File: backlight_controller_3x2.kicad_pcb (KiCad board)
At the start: 2 copper layers, 70.5 x 41.9 mm, 40 parts, among them J1 DB9F_SMD, J2 DB9M_SMD, J3 M12-5-RCPT_F_SMD, J4 M12-5-RCPT_F_SMD, P1 MINI_FIT_JR_02X03_M_RA, U1 SN74ABT541BDWR, U2 SN74ABT541BDWR, U3 NUD3124, U4 NUD3124

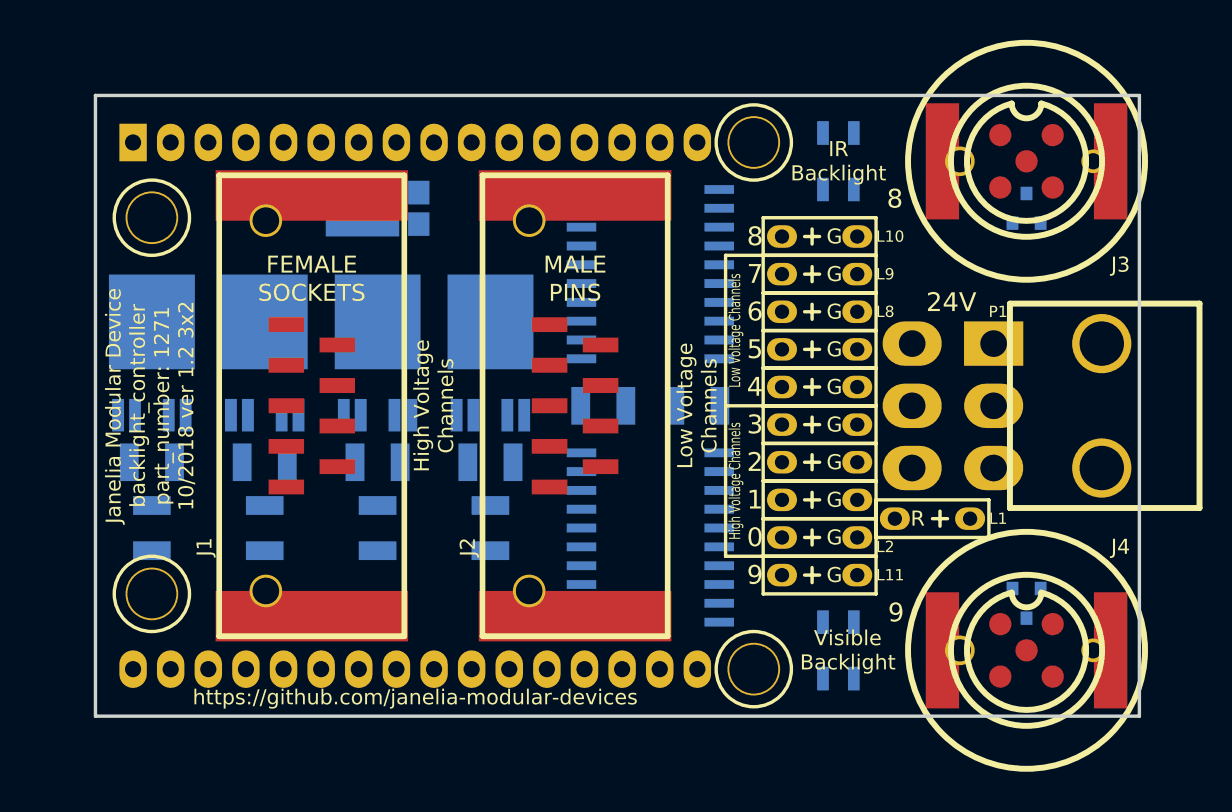
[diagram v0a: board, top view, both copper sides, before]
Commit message: Finished v1.2.
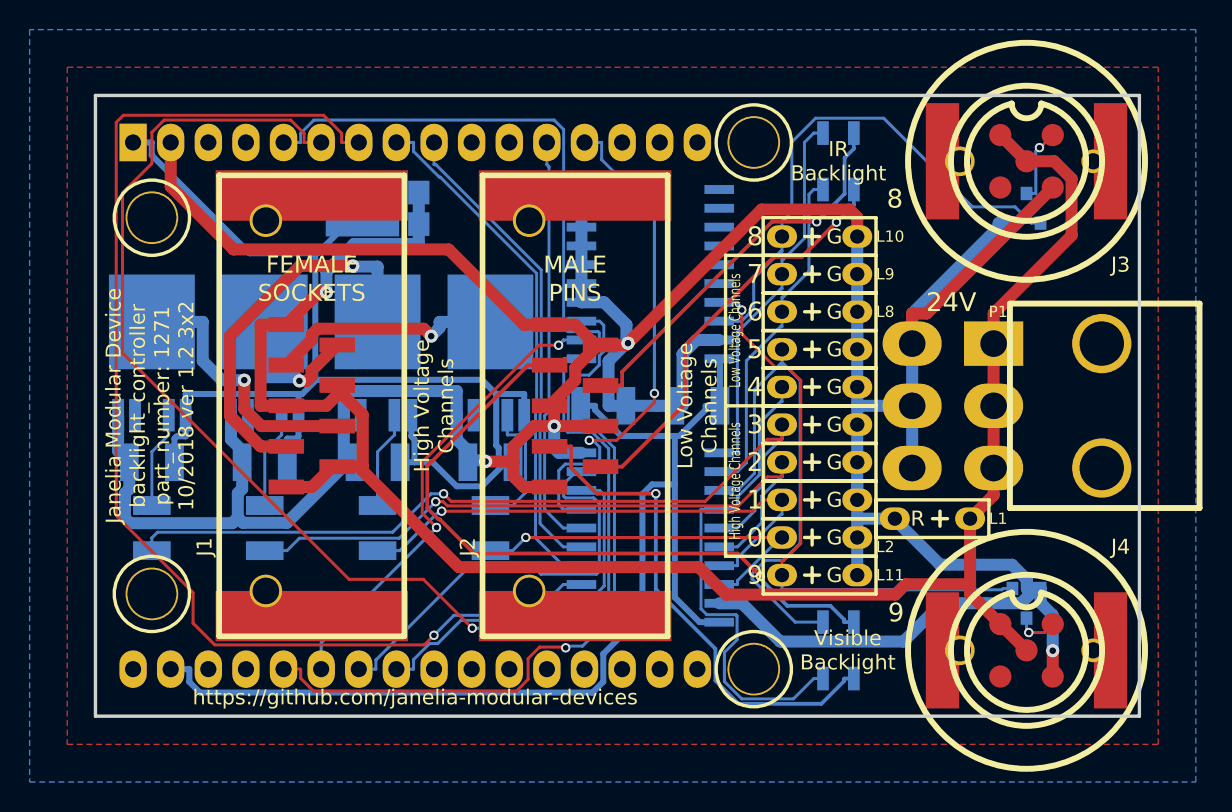
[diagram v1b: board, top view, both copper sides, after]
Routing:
- net GND: track 0.00 -> 271.5 mm, vias 0 -> 4
- net VAA: track 0.00 -> 127.7 mm, vias 0 -> 1
- net /CHANNEL_1: track 0.00 -> 82.2 mm, vias 0 -> 1
- net VDD: track 0.00 -> 82.0 mm
- net VEE: track 0.00 -> 76.1 mm
- net /CHANNEL_0: track 0.00 -> 67.9 mm, vias 0 -> 1
- net /~ENABLE: track 0.00 -> 61.2 mm
- net /backlight_3x2/C_3: track 0.00 -> 57.1 mm, vias 0 -> 1
- net /CHANNEL_9: track 0.00 -> 51.1 mm, vias 0 -> 1
- net /backlight_3x2/C_2: track 0.00 -> 46.4 mm, vias 0 -> 1
- net /backlight_3x2/low_voltage_outputs/OUTPUT_1: track 0.00 -> 46.1 mm, vias 0 -> 1
- net /backlight_3x2/C_9: track 0.00 -> 39.1 mm, vias 0 -> 1
- net /backlight_3x2/C_1: track 0.00 -> 35.7 mm, vias 0 -> 1
- net /backlight_3x2/C_8: track 0.00 -> 35.5 mm
- net /CHANNEL_2: track 0.00 -> 35.2 mm
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- added copper zone on B.Cu, net GND
- added copper zone on F.Cu, net VAA
